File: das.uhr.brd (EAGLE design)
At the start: 95.2 x 36.8 mm, 33 parts, among them CON1 USB-RECEPTABLE, IC1 MCP1700, IC2 MEGA48A-PU, IC3 4017N, IC4 TC4468DP, IC5 TC4468DP, IC6 TC4468DP, IC7 TLC5940-NT, IC8 DCF77, Q1 16M, X3 CATHODES, X4 ANODES, X5 FTDI

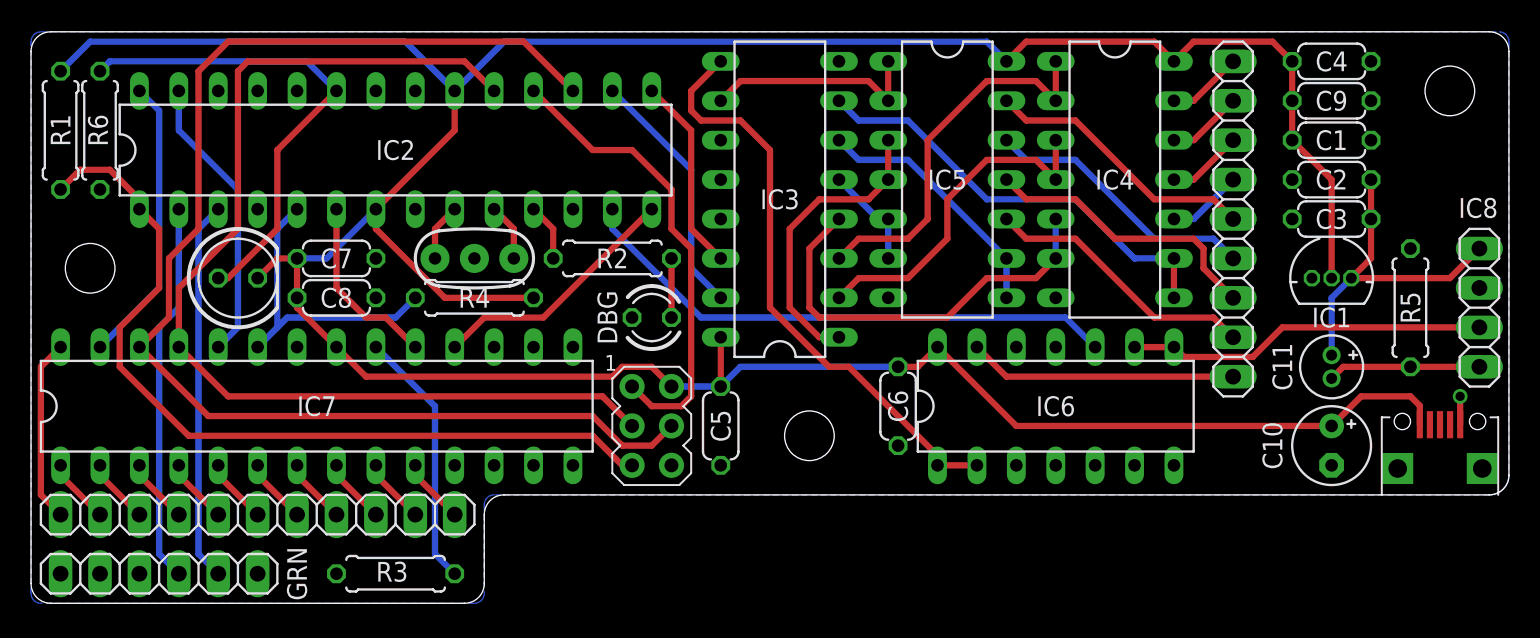
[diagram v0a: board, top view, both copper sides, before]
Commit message: Rev. B1
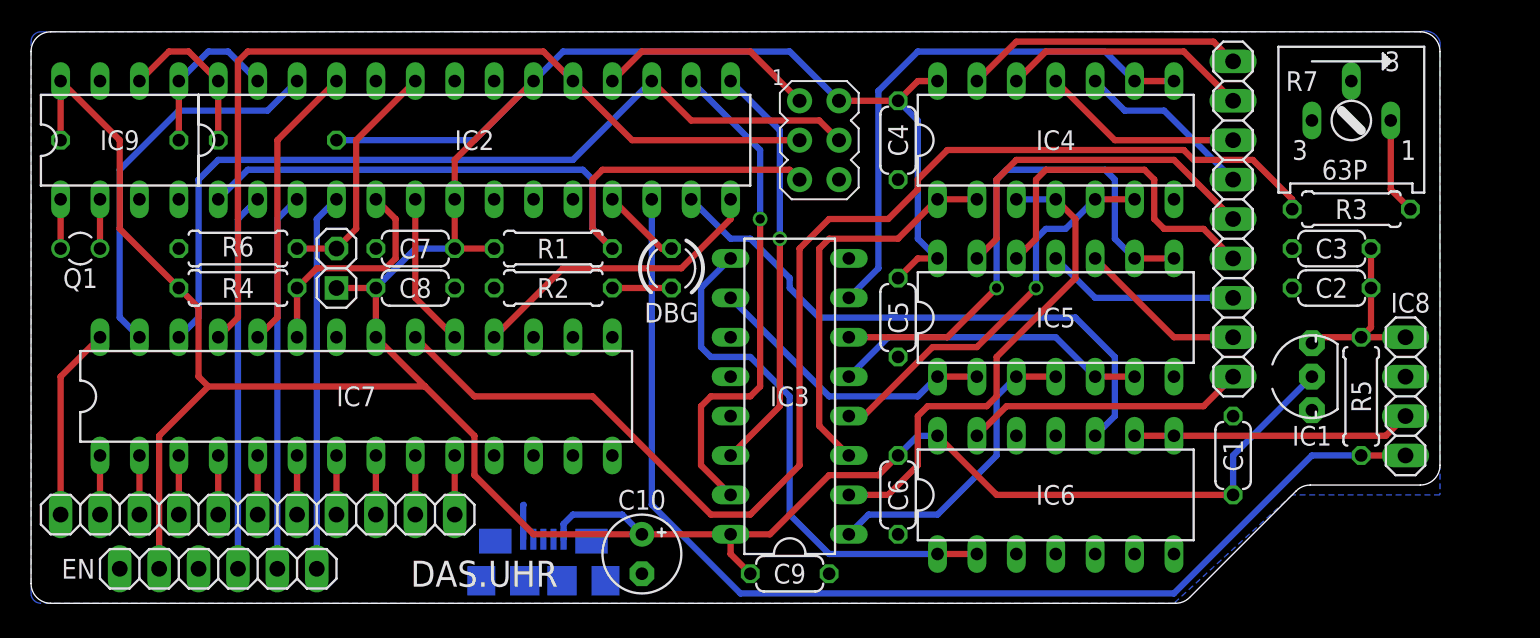
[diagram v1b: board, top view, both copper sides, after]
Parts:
- removed C11: 10µ, daspilker:E1.5-4
- removed U$1: TEPT5700, daspilker:TEPT5700
- removed X5: FTDI, pinhead:1X06
- added CON2: BLUETOOTH, pinhead:1X06
- added IC9: DS1307, daspilker:DIL08
- added R7: 10k, pot:S63P
- added R8: 2.2k, rcl:0207/7
- added R9: 2.2, rcl:0207/7
- added T1: NPN-PHOTOTRANSISTOR-HEADER, daspilker:1X02-S
- CON1: value USB-RECEPTABLE -> PWR; device daspilker:FCI-10103594-0001LF -> daspilker:HIROSE-ZX62-AB-5PA(11)
- IC1: device daspilker:TO92-INLINE-0.5 -> adafruit:TO92-INLINE
- IC2: value MEGA48A-PU -> ATMEGA88PA-PU
- Q1: value 16M -> 32768; device SparkFun:RESONATOR-PTH -> crystal:TC26V
- R3: value 470 -> 330
- moved R3 65.9 mm to (85.1, 25.4), turned to 180 degrees
- moved CON1 58.2 mm to (33.0, 0.00)
- moved C9 46.4 mm to (48.9, 1.91)
- moved C10 45.0 mm to (39.4, 3.17)
- moved R1 32.7 mm to (33.7, 22.9), turned to 180 degrees
- moved C4 28.4 mm to (55.9, 29.8), turned to 270 degrees
- moved Q1 25.4 mm to (3.17, 22.9), turned to 180 degrees
- moved ISP1 21.3 mm to (50.8, 29.8)
- moved C1 21.3 mm to (77.5, 9.53), turned to 90 degrees
- moved R4 15.3 mm to (13.3, 20.3), turned to 180 degrees
- moved C5 13.4 mm to (55.9, 18.4)
- moved IC3 12.7 mm to (48.9, 13.3)
- moved R6 11.7 mm to (13.3, 22.9), turned to 0 degrees
- moved IC5 11.3 mm to (66.0, 18.4), turned to 0 degrees
- moved IC8 7.44 mm to (88.6, 13.3)
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- renumbered X3 to CON3, X4 to CON4
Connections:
- removed net N$12: LED1.A, R2.1
- removed net N$2: IC2.9, Q1.1
- new net BT_EN: CON2.6, IC2.4
- new net N$26: R3.1, R7.A
- new net N$27: IC9.1, Q1.2
- new net N$28: IC9.2, Q1.1
- new net SCL: IC2.28, IC9.6, R8.1
- new net SDA: IC2.27, IC9.5, R9.1
- net +3V3: now also R5.2; no longer C11.+
- net DCF77_PON: now also IC2.12, R5.1; no longer C11.-, R5.2
- net DEBUG_LED: now also LED1.A; no longer R2.2
- net GND: now also CON1.P$5, CON2.3, IC9.3, IC9.4, R2.1, R7.S; no longer CON1.5, LED1.K, Q1.2, R3.1, R5.1
- net N$1: now also LED1.K, R2.2; no longer IC2.10, Q1.3
- net PHOTO: now also T1.2; no longer U$1.E
- net RXD: now also CON2.4; no longer X5.4
- net TXD: now also CON2.5; no longer X5.5
- net VCC: now also CON1.P$1, CON2.2, IC9.8, R8.2, R9.2, T1.1; no longer CON1.1, U$1.C
- net VPRG: now also IC2.26; no longer IC2.28
- net XLAT: now also IC2.25; no longer IC2.27
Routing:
- net N$15: track 16.7 -> 81.5 mm
- net DCF77_PON: track 9.84 -> 74.3 mm
- net SIN/MOSI: track 83.0 -> 56.2 mm
- net BT_EN: track 0.00 -> 24.3 mm
- net ANODES_8: track 16.5 -> 34.1 mm, vias 0 -> 1
- net PHOTO: track 31.9 -> 15.4 mm
- net RES: track 16.2 -> 32.4 mm, vias 0 -> 1
- net MISO: track 30.0 -> 14.2 mm
- net CLK: track 12.6 -> 26.8 mm, vias 0 -> 1
- net ANODES_7: track 6.77 -> 20.5 mm
- net N$24: track 4.86 -> 18.1 mm
- net N$23: track 4.86 -> 16.1 mm
- net SCLK/SCK: track 68.2 -> 57.1 mm
- net SDA: track 0.00 -> 10.5 mm
- net SCL: track 0.00 -> 10.5 mm
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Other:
- board size 95.2 x 36.8 mm -> 90.8 x 36.8 mm
- board text added: "EN"
- board text added: "Rev. B1"
- board text removed: "GRN"
- board text removed: "Rev. A1"
